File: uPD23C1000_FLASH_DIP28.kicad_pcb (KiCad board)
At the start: 2 copper layers, 16.4 x 34.2 mm, 7 parts, among them J1 uPD23C1000, J2 Conn_1x2, J3 Conn_1x3, U1 GLS29EE010 (TSOP), U2 SST39SF010 (TSOP), U3 SST39SF010 / GLS29EE010 (PLCC)

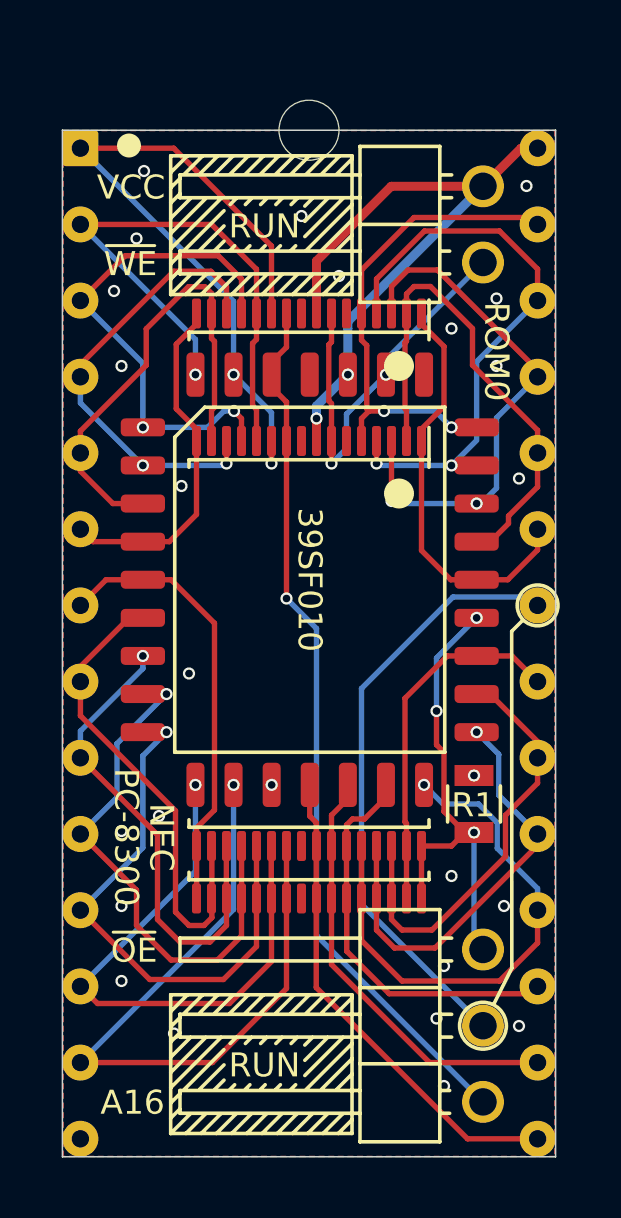
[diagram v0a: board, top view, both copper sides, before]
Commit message: minor tidying
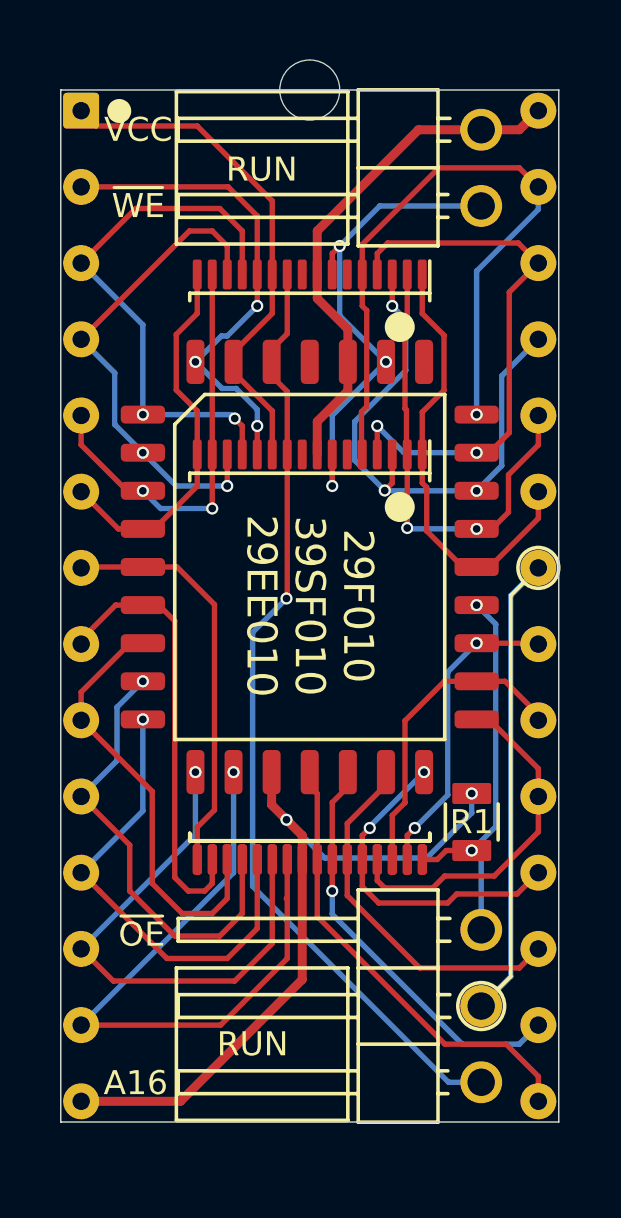
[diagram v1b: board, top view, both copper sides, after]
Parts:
- moved J2 1.89 mm to (155.7, 85.4)
- moved U1 1.30 mm to (150.0, 97.5)
- moved J1 1.25 mm to (150.0, 98.8)
- moved J3 0.66 mm to (155.7, 114.6)
- moved R1 0.60 mm to (155.4, 106.0)
- moved U2 0.45 mm to (150.0, 100.5)
- moved U3 0.42 mm to (150.0, 97.5)
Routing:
- net /GND: track 0.00 -> 24.4 mm, vias 26 -> 2
- net /A15: track 23.9 -> 17.1 mm, vias 2 -> 0
- net /D6: track 17.8 -> 11.2 mm, vias 1 -> 2
- net /A14: track 16.4 -> 22.3 mm, vias 2 -> 1
- net /A16_OE: track 20.2 -> 15.4 mm
- net /VCC: track 21.5 -> 17.4 mm, vias 2 -> 0
- net /~CE: track 14.4 -> 10.4 mm
- net /~WE: track 13.9 -> 16.8 mm, vias 2 -> 3
- net /D0: track 18.5 -> 15.7 mm
- net /A0: track 17.8 -> 15.0 mm
- net /D7: track 14.5 -> 11.8 mm, vias 1 -> 0
- net /A12: track 18.8 -> 16.3 mm, vias 1 -> 3
- net /~OE: track 15.8 -> 13.3 mm, vias 3 -> 2
- net /D2: track 24.0 -> 21.6 mm
- net /A16: track 29.4 -> 31.6 mm
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- removed copper zone on B.Cu, net /GND
- removed copper zone on F.Cu, net /GND
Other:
- board size 16.4 x 34.2 mm -> 16.6 x 34.4 mm
- board text added: "29F010 39SF010 29EE010"
- board text added: "29F010 to uPD23C1000"
- board text added: "Move the A16 jumper to ~OE~"
- board text added: "Remove the VCC/~WE~ jumper"
- board text added: "Set programmer for installed chip (ex: SST39SF010 not uPD23C1000)"
- board text added: "github.com/bkw777/aDIPters"
- board text removed: "39SF010"
- board text removed: "Configure programmer for PLCC version of chip (even if chip is TSOP)"
- board text removed: "Move A16 jumper to ~OE~"
- board text removed: "NEC"
- board text removed: "NEC PC-8300 System ROM"
- board text removed: "PC-8300"
- board text removed: "ROM0"
- board text removed: "Remove VCC/~WE~ jumper"
- board text removed: "http://tandy.wiki/FlashROM_8300"
